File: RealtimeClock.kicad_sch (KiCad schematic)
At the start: 6 parts, among them U21 74HC02, U22 DS12885+, Y2 32.768kHz

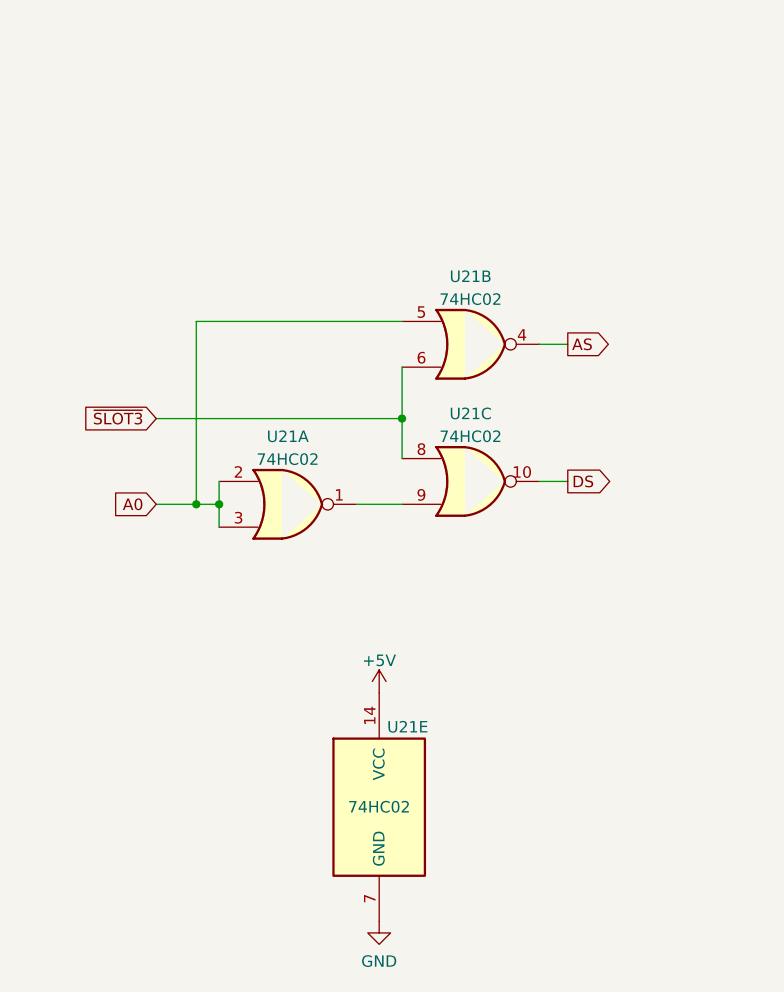
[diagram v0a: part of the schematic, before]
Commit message: Schematic cleanup
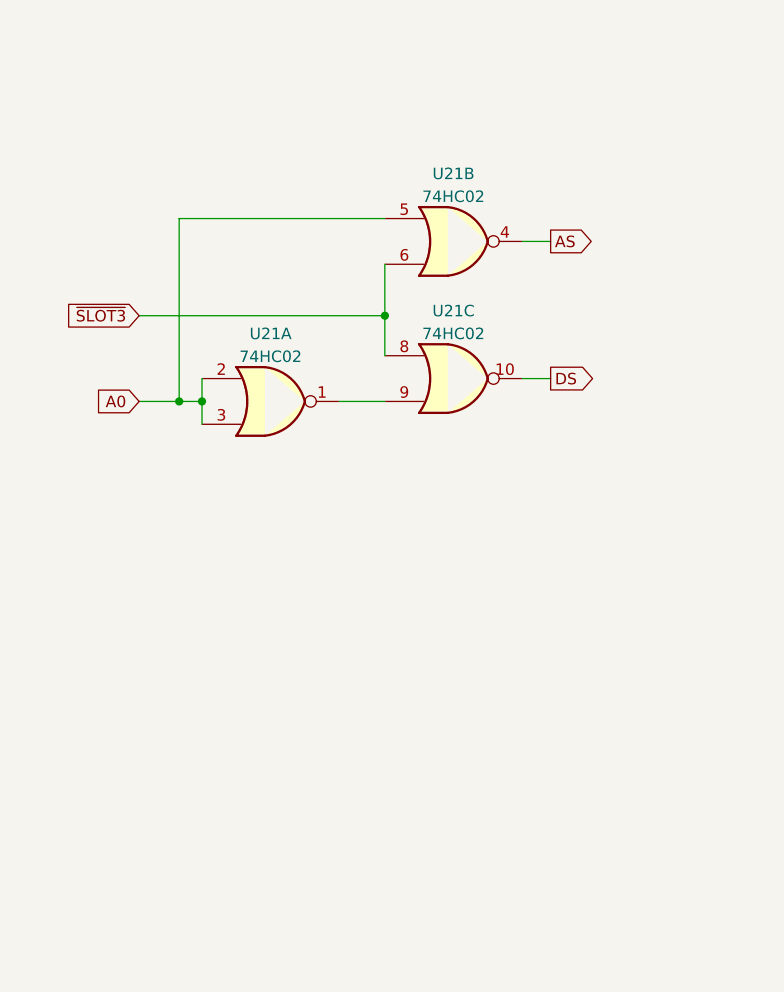
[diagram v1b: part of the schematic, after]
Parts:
- removed unit 5 of U21
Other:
- moved on the sheet: U21A, U21B, U21C
